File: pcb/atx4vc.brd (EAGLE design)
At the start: 69.4 x 69 mm, 52 parts, among them IC1 MY_7905DT, J2 ATX24RH

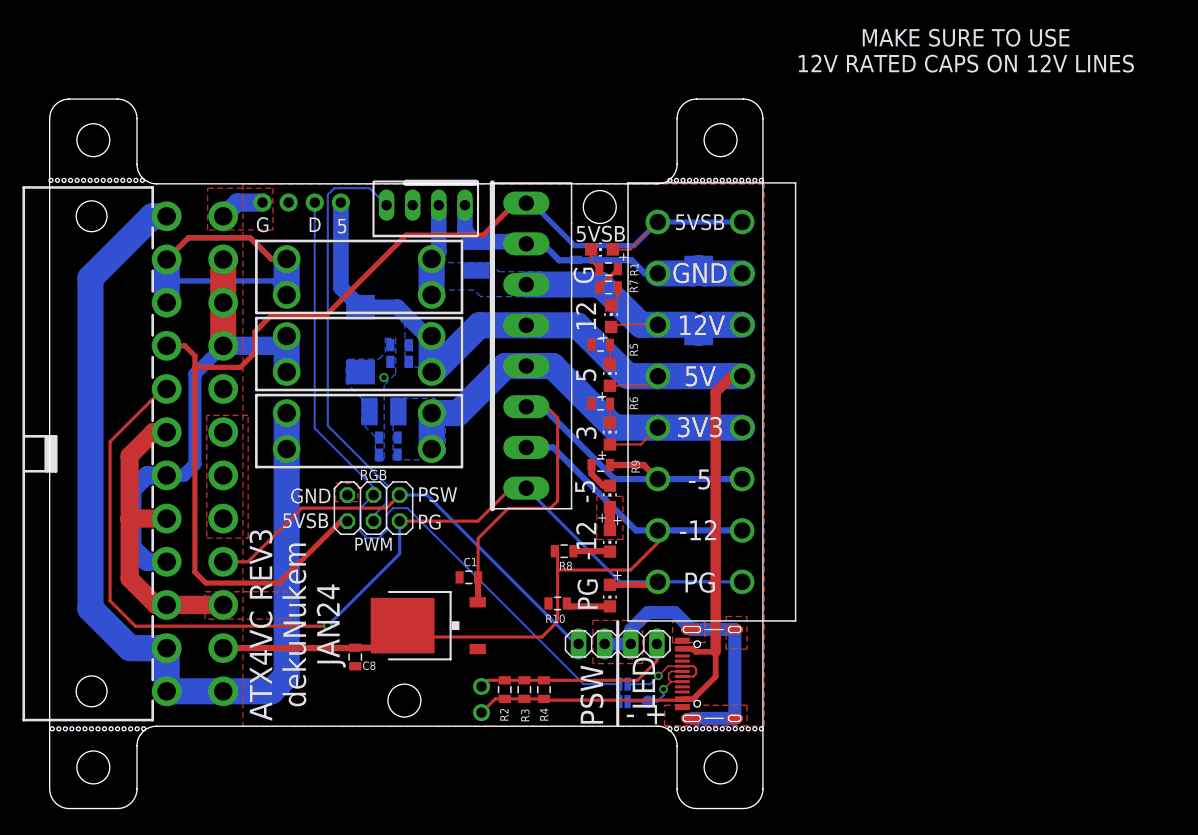
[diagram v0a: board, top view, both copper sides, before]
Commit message: equal dimension
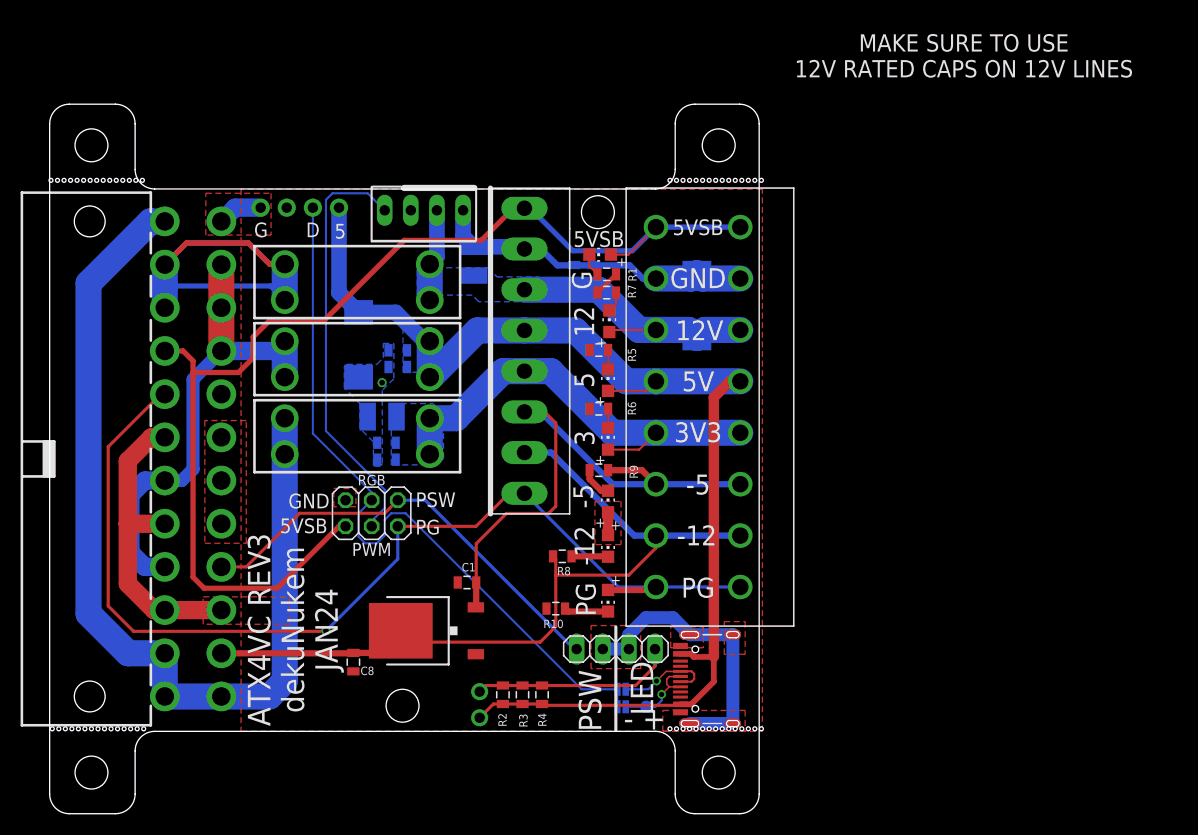
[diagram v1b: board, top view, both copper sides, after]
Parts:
- moved C1 0.53 mm to (40.6, 22.5)
- moved C11 0.53 mm to (41.2, 53.7)
- moved C4 0.53 mm to (33.9, 45.1)
- moved C5 0.53 mm to (33.9, 43.4)
- moved LED2 0.53 mm to (54.3, 42.2)
- moved LED6 0.53 mm to (54.3, 30.4)
- moved R1 0.53 mm to (54.2, 52.5)
- moved R3 0.53 mm to (46.0, 11.6)
- moved R4 0.53 mm to (47.9, 11.6)
- moved R5 0.53 mm to (53.4, 45.1)
- moved R6 0.53 mm to (53.4, 39.4)
- moved R7 0.53 mm to (54.2, 50.7)
- moved R9 0.53 mm to (53.4, 33.4)
- moved TP1 0.53 mm to (58.0, 10.4)
- moved U$12 0.53 mm to (63.1, 42.0)
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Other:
- board size 69.4 x 69 mm -> 69 x 69 mm
